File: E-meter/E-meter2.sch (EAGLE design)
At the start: 32 parts, among them IC1 LM324N, IC2 7805T

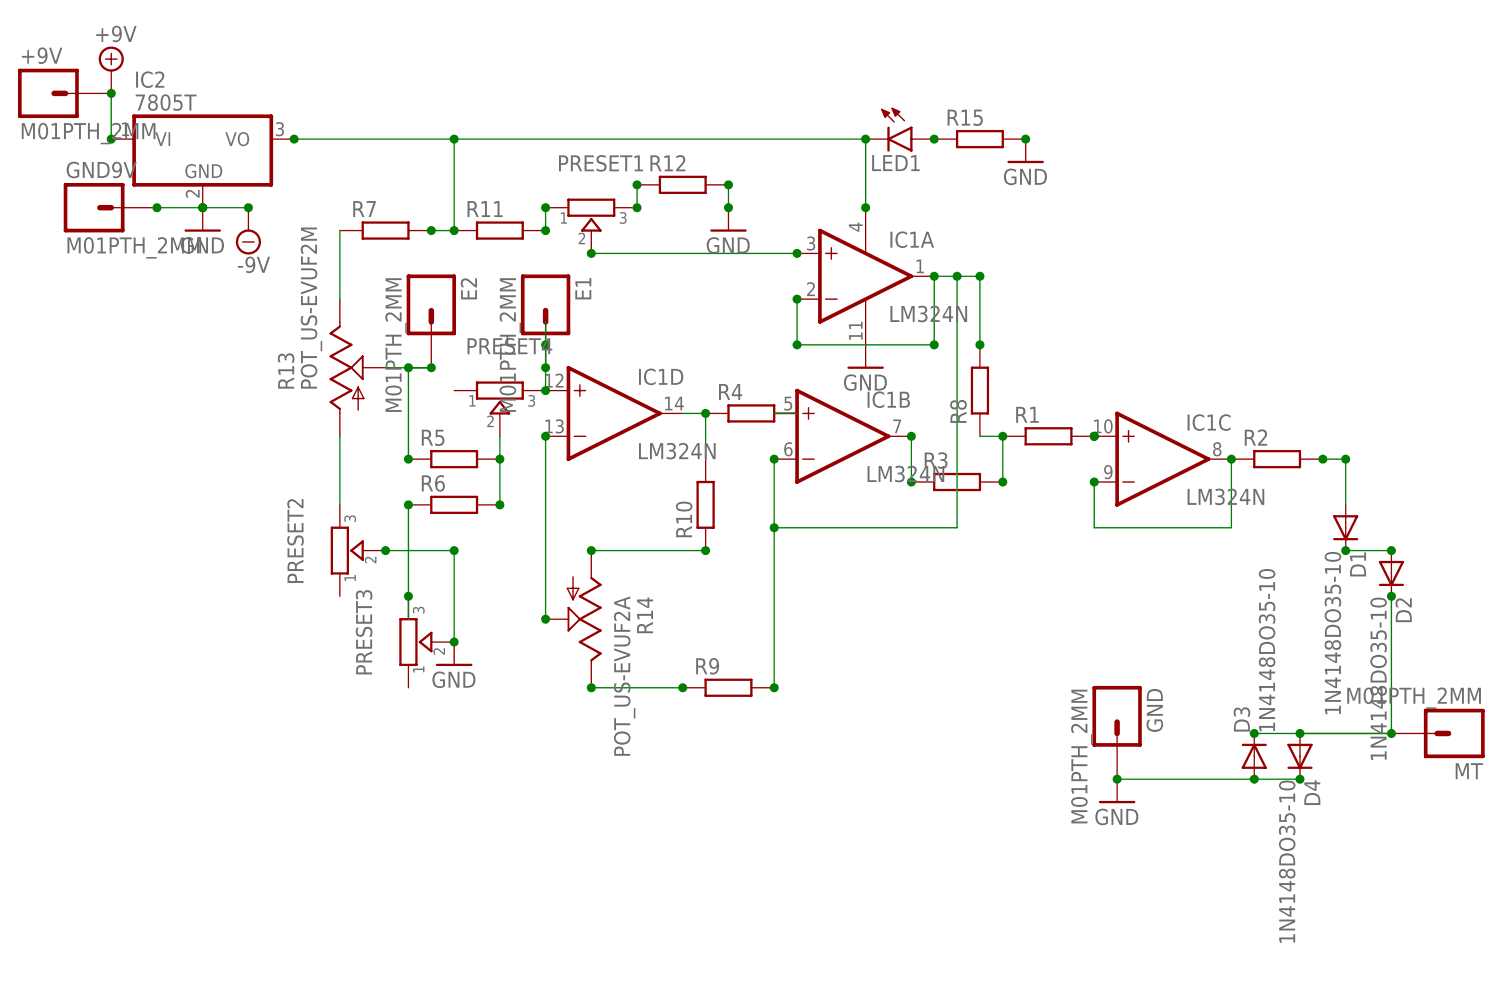
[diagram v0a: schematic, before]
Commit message: new layout
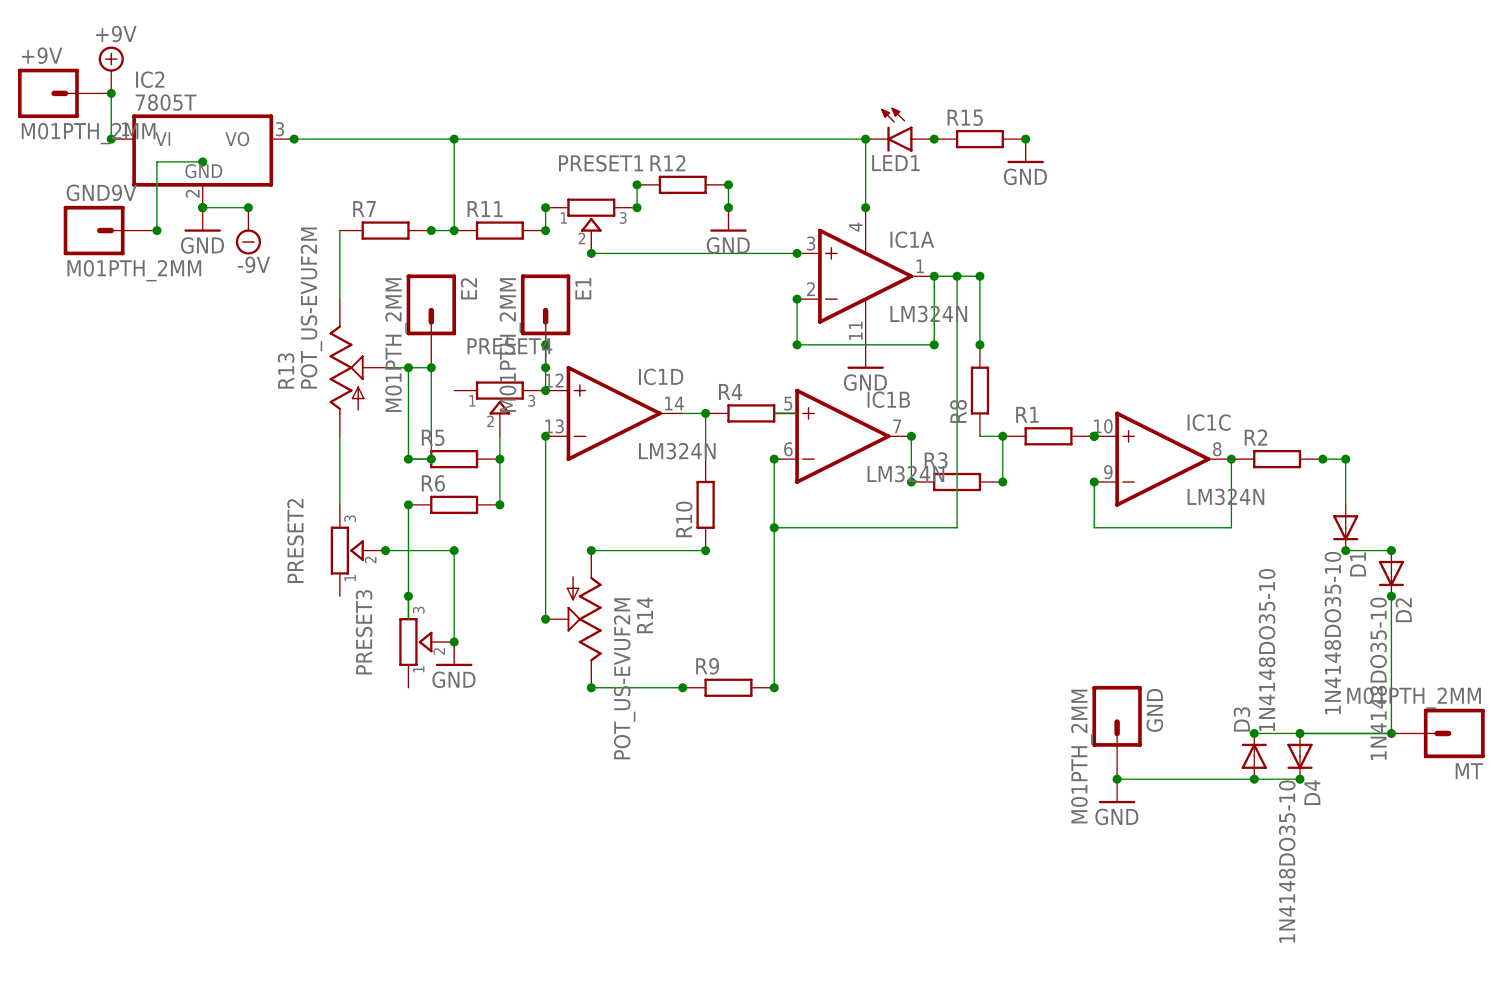
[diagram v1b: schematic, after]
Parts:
- R14: value POT_US-EVUF2A -> POT_US-EVUF2M; device 4009dist_PWM3_v1:POT_US-EVUF2A -> 4009dist_PWM3_v1:POT_US-EVUF2M
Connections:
- new net N$18: GND9V.1
- net GND: no longer GND9V.1
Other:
- moved on the sheet: GND9V
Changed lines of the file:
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@@
 <grid distance="0.1" unitdist="inch" unit="inch" style="lines" multiple="1" display="no" altdistance="0.01" altunitdist="inch" altunit="inch"/>
 <layers>
-<layer number="1" name="Top" color="4" fill="1" visible="no" active="no"/>
-<layer number="16" name="Bottom" color="1" fill="1" visible="no" active="no"/>
-<layer number="17" name="Pads" color="2" fill="1" visible="no" active="no"/>
-<layer number="18" name="Vias" color="2" fill="1" visible="no" active="no"/>
-<layer number="19" name="Unrouted" color="6" fill="1" visible="no" active="no"/>
-<layer number="20" name="Dimension" color="15" fill="1" visible="no" active="no"/>
-<layer number="21" name="tPlace" color="7" fill="1" visible="no" active="no"/>
-<layer number="22" name="bPlace" color="7" fill="1" visible="no" active="no"/>
-<layer number="23" name="tOrigins" color="15" fill="1" visible="no" active="no"/>
-<layer number="24" name="bOrigins" color="15" fill="1" visible="no" active="no"/>
-<layer number="25" name="tNames" color="7" fill="1" visible="no" active="no"/>
-<layer number="26" name="bNames" color="7" fill="1" visible="no" active="no"/>
-<layer number="27" name="tValues" color="7" fill="1" visible="no" active="no"/>
-<layer number="28" name="bValues" color="7" fill="1" visible="no" active="no"/>
+<layer number="1" name="Top" color="4" fill="1" visible="yes" active="no"/>
+<layer number="16" name="Bottom" color="1" fill="1" visible="yes" active="no"/>
+<layer number="17" name="Pads" color="2" fill="1" visible="yes" active="no"/>
+<layer number="18" name="Vias" color="2" fill="1" visible="yes" active="no"/>
+<layer number="19" name="Unrouted" color="6" fill="1" visible="yes" active="no"/>
+<layer number="20" name="Dimension" color="15" fill="1" visible="yes" active="no"/>
+<layer number="21" name="tPlace" color="7" fill="1" visible="yes" active="no"/>
+<layer number="22" name="bPlace" color="7" fill="1" visible="yes" active="no"/>
+<layer number="23" name="tOrigins" color="15" fill="1" visible="yes" active="no"/>
+<layer number="24" name="bOrigins" color="15" fill="1" visible="yes" active="no"/>
+<layer number="25" name="tNames" color="7" fill="1" visible="yes" active="no"/>
+<layer number="26" name="bNames" color="7" fill="1" visible="yes" active="no"/>
+<layer number="27" name="tValues" color="7" fill="1" visible="yes" active="no"/>
+<layer number="28" name="bValues" color="7" fill="1" visible="yes" active="no"/>
 <layer number="29" name="tStop" color="7" fill="3" visible="no" active="no"/>
 <layer number="30" name="bStop" color="7" fill="6" visible="no" active="no"/>
@@
 <layer number="35" name="tGlue" color="7" fill="4" visible="no" active="no"/>
 <layer number="36" name="bGlue" color="7" fill="5" visible="no" active="no"/>
-<layer number="37" name="tTest" color="7" fill="1" visible="no" active="no"/>
-<layer number="38" name="bTest" color="7" fill="1" visible="no" active="no"/>
+<layer number="37" name="tTest" color="7" fill="1" visible="yes" active="no"/>
+<layer number="38" name="bTest" color="7" fill="1" visible="yes" active="no"/>
 <layer number="39" name="tKeepout" color="4" fill="11" visible="no" active="no"/>
 <layer number="40" name="bKeepout" color="1" fill="11" visible="no" active="no"/>
@@
 <layer number="44" name="Drills" color="7" fill="1" visible="no" active="no"/>
 <layer number="45" name="Holes" color="7" fill="1" visible="no" active="no"/>
-<layer number="46" name="Milling" color="3" fill="1" visible="no" active="no"/>
-<layer number="47" name="Measures" color="7" fill="1" visible="no" active="no"/>
-<layer number="48" name="Document" color="7" fill="1" visible="no" active="no"/>
-<layer number="49" name="Reference" color="7" fill="1" visible="no" active="no"/>
-<layer number="50" name="dxf" color="7" fill="1" visible="no" active="no"/>
-<layer number="51" name="tDocu" color="7" fill="1" visible="no" active="no"/>
-<layer number="52" name="bDocu" color="7" fill="1" visible="no" active="no"/>
-<layer number="53" name="tGND_GNDA" color="7" fill="1" visible="no" active="no"/>
-<layer number="54" name="bGND_GNDA" color="7" fill="1" visible="no" active="no"/>
-<layer number="56" name="wert" color="7" fill="1" visible="no" active="no"/>
-<layer number="57" name="tCAD" color="7" fill="1" visible="no" active="no"/>
+<layer number="46" name="Milling" color="3" fill="1" visible="yes" active="no"/>
+<layer number="47" name="Measures" color="7" fill="1" visible="yes" active="no"/>
+<layer number="48" name="Document" color="7" fill="1" visible="yes" active="no"/>
+<layer number="49" name="Reference" color="7" fill="1" visible="yes" active="no"/>
+<layer number="50" name="dxf" color="7" fill="1" visible="yes" active="no"/>
+<layer number="51" name="tDocu" color="7" fill="1" visible="yes" active="no"/>
+<layer number="52" name="bDocu" color="7" fill="1" visible="yes" active="no"/>
+<layer number="53" name="tGND_GNDA" color="7" fill="1" visible="yes" active="no"/>
+<layer number="54" name="bGND_GNDA" color="7" fill="1" visible="yes" active="no"/>
+<layer number="56" name="wert" color="7" fill="1" visible="yes" active="no"/>
+<layer number="57" name="tCAD" color="7" fill="1" visible="yes" active="no"/>
 <layer number="90" name="Modules" color="5" fill="1" visible="yes" active="yes"/>
 <layer number="91" name="Nets" color="2" fill="1" visible="yes" active="yes"/>
@@
 <part name="PRESET3" library="dp_devices" deviceset="TRIMMER" device="-3306F"/>
 <part name="PRESET4" library="dp_devices" deviceset="TRIMMER" device="-3306F"/>
-<part name="R14" library="4009dist_PWM3_v1" deviceset="POT_US-EVU" device="A" technology="F2"/>
+<part name="R14" library="4009dist_PWM3_v1" deviceset="POT_US-EVU" device="M" technology="F2" value="POT_US-EVUF2M"/>
 <part name="IC2" library="linear" deviceset="78*" device="T" technology="05"/>
 <part name="GND1" library="supply1" deviceset="GND" device=""/>
@@
 <instance part="MT" gate="G$1" x="134.62" y="7.62" rot="R180"/>
 <instance part="GND" gate="G$1" x="96.52" y="10.16" rot="R270"/>
-<instance part="GND9V" gate="G$1" x="-17.78" y="66.04"/>
+<instance part="GND9V" gate="G$1" x="-17.78" y="63.5"/>
 <instance part="+9V" gate="G$1" x="-22.86" y="78.74"/>
 <instance part="LED1" gate="G$1" x="73.66" y="73.66" rot="R270"/>
@@
 <pinref part="SUPPLY2" gate="G$1" pin="-9V"/>
 <wire x1="0" y1="66.04" x2="-5.08" y2="66.04" width="0.1524" layer="91"/>
-<pinref part="GND9V" gate="G$1" pin="1"/>
-<wire x1="-10.16" y1="66.04" x2="-5.08" y2="66.04" width="0.1524" layer="91"/>
-<junction x="-10.16" y="66.04"/>
 <junction x="0" y="66.04"/>
 </segment>
@@
 <pinref part="R13" gate="G$1" pin="S"/>
 <pinref part="R5" gate="G$1" pin="1"/>
-<wire x1="20.32" y1="48.26" x2="17.78" y2="48.26" width="0.1524" layer="91"/>
-<wire x1="17.78" y1="48.26" x2="17.78" y2="38.1" width="0.1524" layer="91"/>
 <junction x="17.78" y="38.1"/>
 <junction x="20.32" y="48.26"/>
 <pinref part="E2" gate="G$1" pin="1"/>
-<wire x1="20.32" y1="48.26" x2="17.78" y2="48.26" width="0.1524" layer="91"/>
 <junction x="17.78" y="48.26"/>
 <wire x1="17.78" y1="48.26" x2="15.24" y2="48.26" width="0.1524" layer="91"/>
+<wire x1="20.32" y1="48.26" x2="17.78" y2="48.26" width="0.1524" layer="91"/>
+<wire x1="17.78" y1="48.26" x2="17.78" y2="38.1" width="0.1524" layer="91"/>
+<wire x1="20.32" y1="48.26" x2="20.32" y2="38.1" width="0.1524" layer="91"/>
+<wire x1="20.32" y1="38.1" x2="17.78" y2="38.1" width="0.1524" layer="91"/>
+<junction x="20.32" y="38.1"/>
 </segment>
 </net>
@@
 </segment>
 </net>
+<net name="N$18" class="0">
+<segment>
+<pinref part="GND9V" gate="G$1" pin="1"/>
+<wire x1="-5.08" y1="71.12" x2="-10.16" y2="71.12" width="0.1524" layer="91"/>
+<wire x1="-10.16" y1="71.12" x2="-10.16" y2="63.5" width="0.1524" layer="91"/>
+<junction x="-10.16" y="63.5"/>
+<junction x="-5.08" y="71.12"/>
+</segment>
+</net>
